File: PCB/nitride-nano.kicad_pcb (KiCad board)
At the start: 6 copper layers, 120 x 57 mm, 315 parts, among them J3 XT-90-M, J4 SWD, J5 SSD1306, J6 XT90-F, P1 USB_C_Plug_USB2.0, Q1 EPC2367, Q10 SQJB90EP-T1_GE3, Q12 AO3400A, Q13 AO3404A, Q2 EPC2367, Q3 EPC2367, Q4 EPC2367, Q5 EPC2367, Q6 AGM612AP, Q7 AO3401A, Q8 AO3404A, Q9 AO3404A, SW1 EC11E15244G1, SW2 KMR211NGLFS, SW3 KMR211NGLFS, U1 LT8390AIUFD-PBF, U11 LMR16006XDDCR, U12 INA228AIDGSR, U13 LMR16006XDDCR, U14 INA241A1xDDF, U2 STM32G474CEUx, U3 TPD4S480RUKR, U4 TPS26750SRSMR, U5 LM2765, U6 CAT24C512YI-GT3, U7 TMUX1574RSV, U8 LTC7004x, U9 INA228AIDGSR, Y1 8M

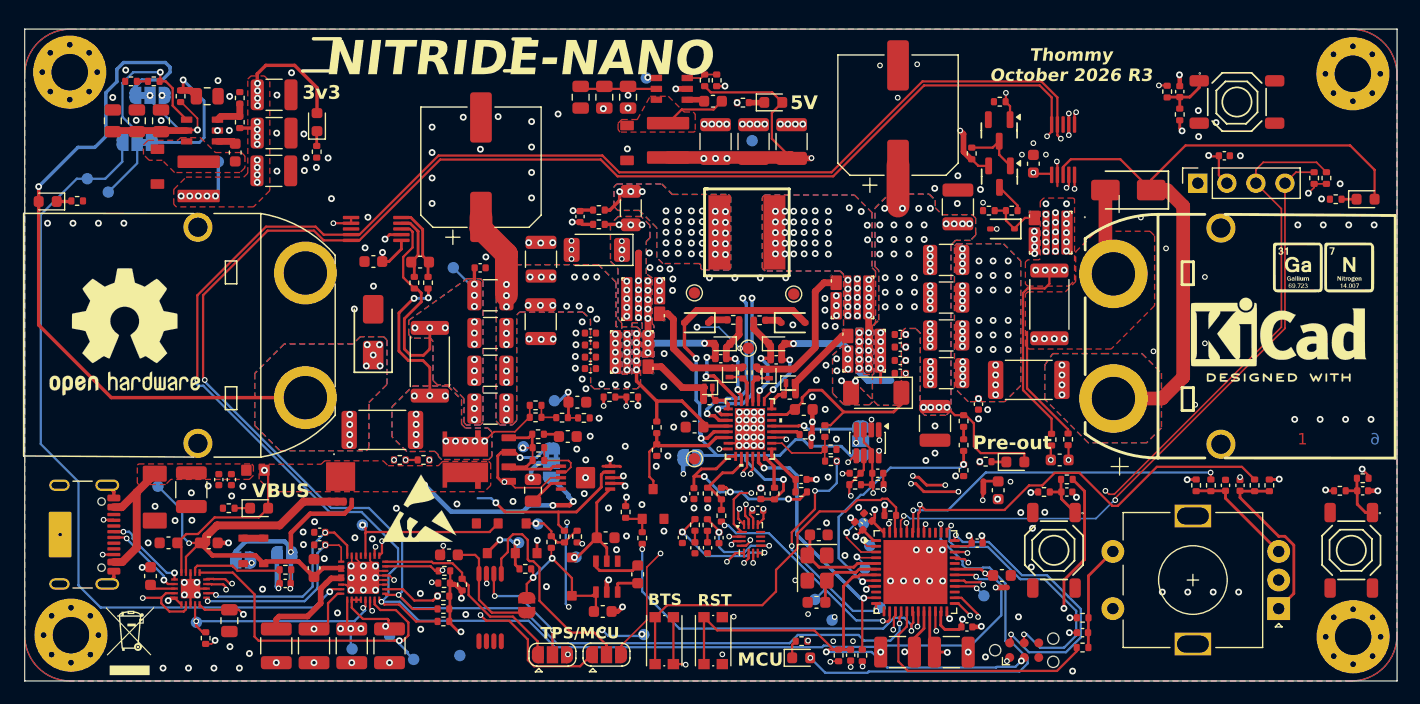
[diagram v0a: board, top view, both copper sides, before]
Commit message: Housing Rev3 added
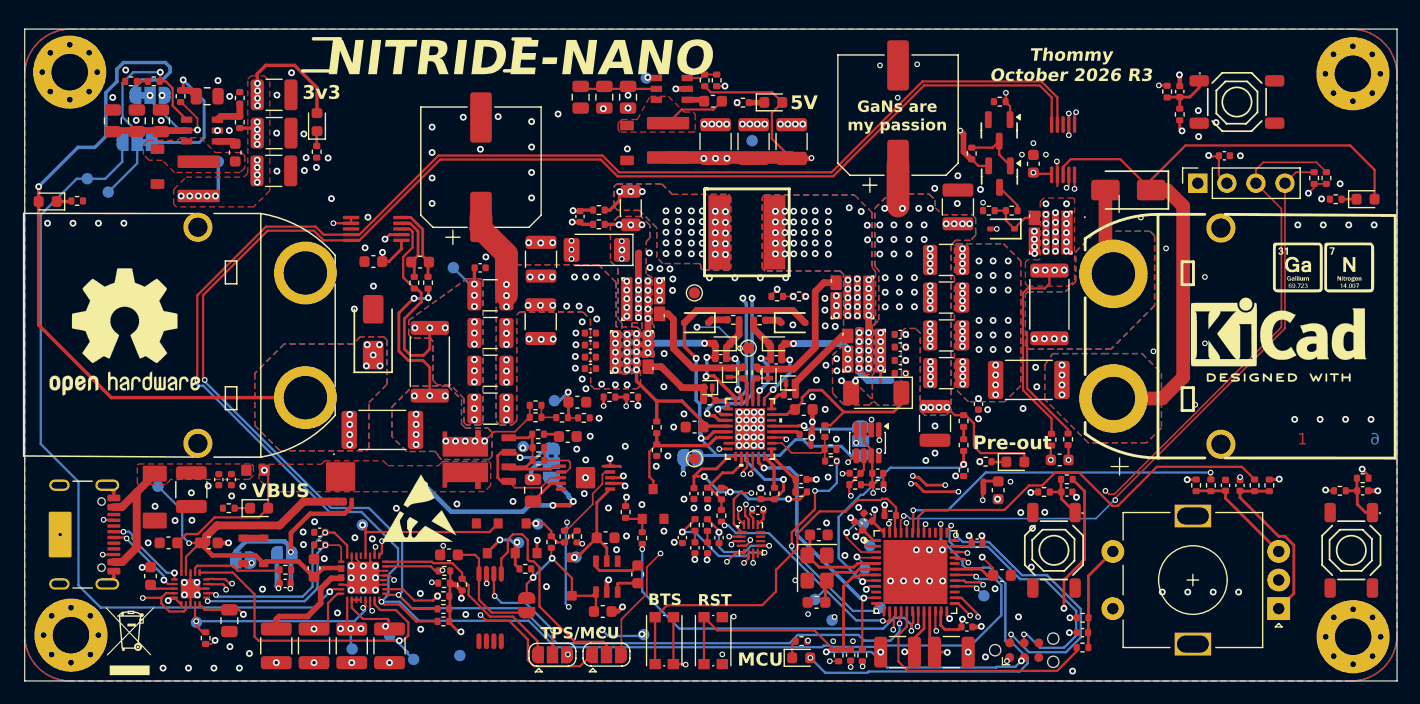
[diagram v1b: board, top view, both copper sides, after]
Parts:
- removed NT1: nt_2pad_20x20_20_60x20, Altium_port:NetTie-2_SMD_Pad0.5mm
- removed TP35: tp_round_70, TestPoint:TestPoint_Pad_D1.0mm
- moved R51 37.7 mm to (103.4, 88.7), turned to 0 degrees
- moved R50 34.1 mm to (101.5, 88.7), turned to 0 degrees
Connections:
- R51 pad 2: Net-(NT1-Pad1) -> GND
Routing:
- net Net-(NT1-Pad1): track 59.5 -> 0.00 mm, vias 2 -> 0
- net /MCU/Temp PWR In: track 60.4 -> 40.9 mm
- net Net-(U8-INP): track 16.3 -> 7.15 mm, vias 1 -> 0
- net /MCU/I2C0_SDA: track 195.7 -> 194.3 mm, vias 4 -> 3
- net +3V3: track 79.1 -> 80.0 mm
- net /MCU/ENC_A: track 36.4 -> 35.5 mm, vias 1 -> 0
- net /MCU/I2C0_SCL: track 176.5 -> 176.0 mm, vias 4 -> 3
- net GND: track 94.3 -> 94.5 mm, vias 321 -> 329
- net /USB-PD/TS: vias 2 -> 1
- added copper zone on B.Cu, net /Power-Sense-Out/PWR-In
- added copper zone on In3.Cu, net /Power-Sense-Out/PWR-In
- added copper zone on In4.Cu, net /Power-Sense-Out/PWR-In
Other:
- board text added: "GaNs are my passion"
- board text added: "LY Wicky"
